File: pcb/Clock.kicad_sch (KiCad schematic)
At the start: 19 parts, among them Y3 Si5351C-B-GM, Y4 3225-25M-SR

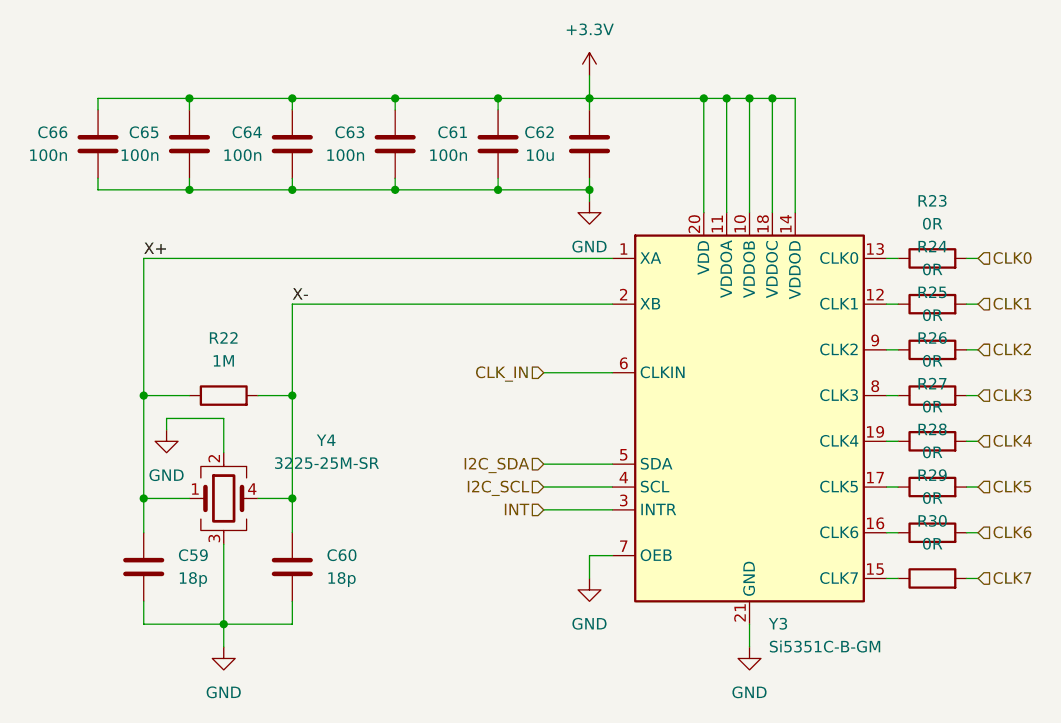
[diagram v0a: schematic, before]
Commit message: Clock rounting
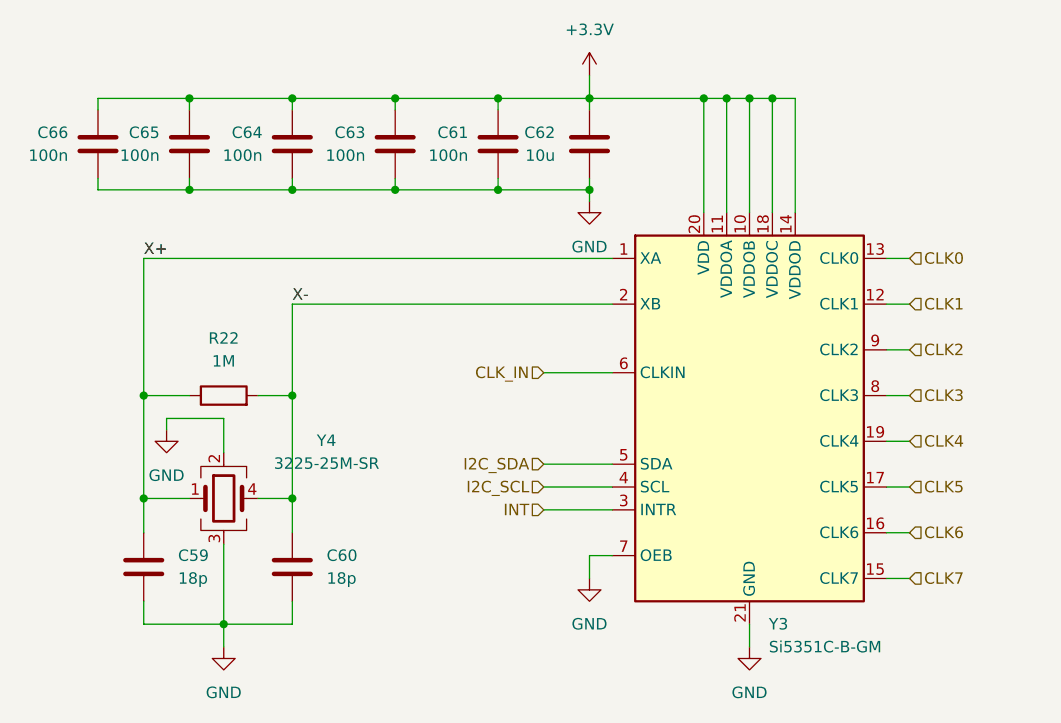
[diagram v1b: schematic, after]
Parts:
- removed R23, R24, R25, R26, R27, R28, R29, R30: 0R, Resistor_SMD:R_0402_1005Metric_Pad0.72x0.64mm_HandSolder, symbol Device:R
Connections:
- net CLK0: now also Y3.13 (CLK0)
- net CLK1: now also Y3.12 (CLK1)
- net CLK2: now also Y3.9 (CLK2)
- net CLK3: now also Y3.8 (CLK3)
- net CLK4: now also Y3.19 (CLK4)
- net CLK5: now also Y3.17 (CLK5)
- net CLK6: now also Y3.16 (CLK6)
- net CLK7: now also Y3.15 (CLK7)
